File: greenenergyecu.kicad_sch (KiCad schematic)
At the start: 4 parts, among them M1 Module-vr-discrete-0.5, M2 Module-knock-0.2, M3 Module-vr-0.1, M4 Module-motor-driver-0.1

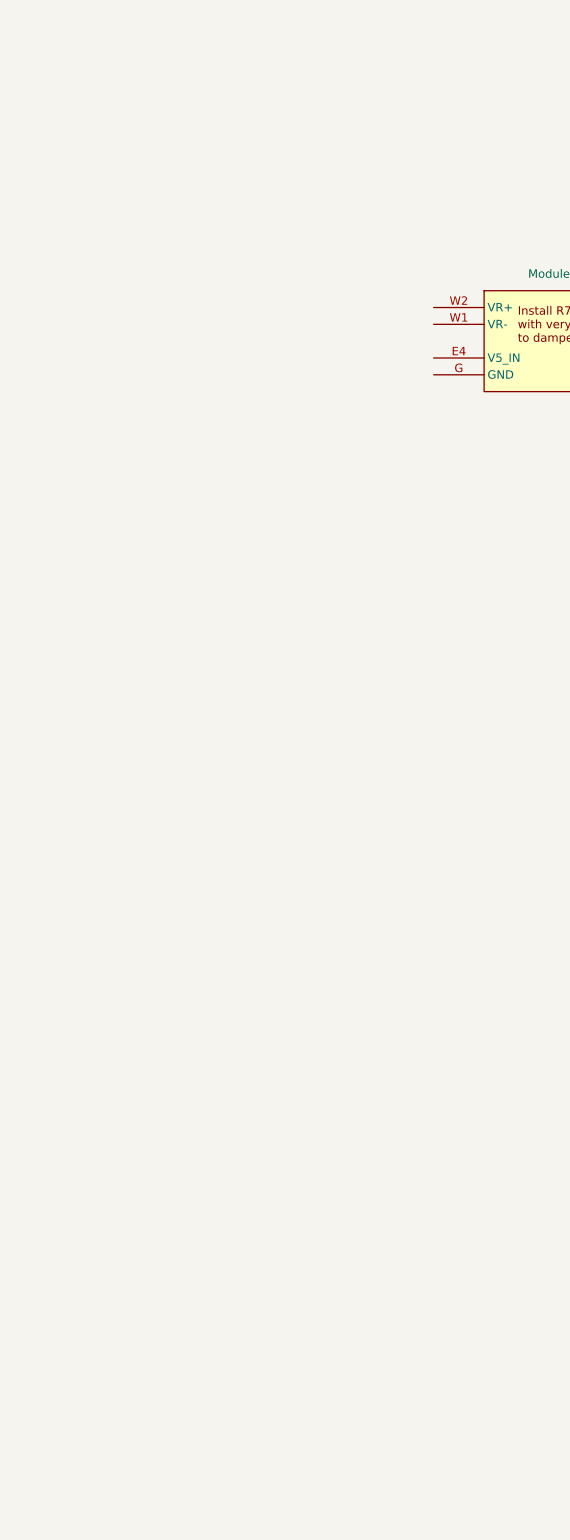
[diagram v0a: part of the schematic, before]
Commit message: ew
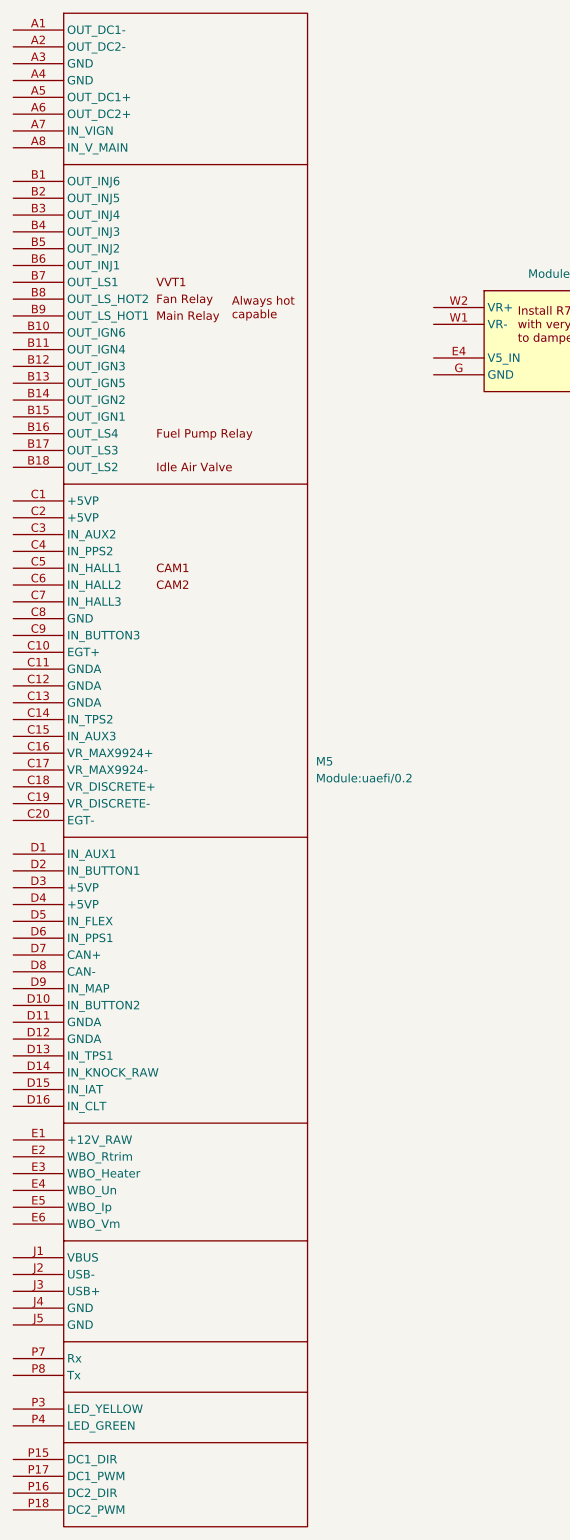
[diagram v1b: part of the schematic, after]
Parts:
- added M5: Module:uaefi/0.2, 0.2:uaefi, symbol uaefi:Module-uaefi-0.2
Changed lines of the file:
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@@
+	)
+	(symbol
+		(lib_id "uaefi:Module-uaefi-0.2")
+		(at -25.4 -3.81 0)
+		(unit 1)
+		(exclude_from_sim no)
+		(in_bom yes)
+		(on_board yes)
+		(dnp no)
+		(fields_autoplaced yes)
+		(property "Reference" "M5"
+			(at 20.32 106.6799 0)
+			(effects
+				(font
+					(size 1.27 1.27)
+				)
+				(justify left)
+			)
+		)
+		(property "Value" "Module:uaefi/0.2"
+			(at 20.32 109.2199 0)
+			(effects
+				(font
+					(size 1.27 1.27)
+				)
+				(justify left)
+			)
+		)
+		(property "Footprint" "0.2:uaefi"
+			(at -3.81 223.52 0)
+			(effects
+				(font
+					(size 1.27 1.27)
+				)
+				(hide yes)
+			)
+		)
+		(property "Datasheet" ""
+			(at -25.4 -3.81 0)
+			(effects
+				(font
+					(size 1.27 1.27)
+				)
+				(hide yes)
+			)
+		)
+		(property "Description" ""
+			(at -25.4 -3.81 0)
+			(effects
+				(font
+					(size 1.27 1.27)
+				)
+				(hide yes)
+			)
+		)
+		(pin "D12"
+		)
+		(pin "D14"
+		)
+		(pin "A1"
+		)
+		(pin "D15"
+		)
+		(pin "A6"
+		)
+		(pin "B1"
+		)
+		(pin "B11"
+		)
+		(pin "E1"
+		)
+		(pin "C17"
+		)
+		(pin "A3"
+		)
+		(pin "B16"
+		)
+		(pin "C16"
+		)
+		(pin "E2"
+		)
+		(pin "E5"
+		)
+		(pin "E6"
+		)
+		(pin "E3"
+		)
+		(pin "A7"
+		)
+		(pin "P4"
+		)
+		(pin "D3"
+		)
+		(pin "C15"
+		)
+		(pin "D4"
+		)
+		(pin "P18"
+		)
+		(pin "D8"
+		)
+		(pin "D10"
+		)
+		(pin "D16"
+		)
+		(pin "D9"
+		)
+		(pin "D6"
+		)
+		(pin "D5"
+		)
+		(pin "D7"
+		)
+		(pin "E4"
+		)
+		(pin "J1"
+		)
+		(pin "A4"
+		)
+		(pin "J3"
+		)
+		(pin "J4"
+		)
+		(pin "P16"
+		)
+		(pin "D1"
+		)
+		(pin "C19"
+		)
+		(pin "P17"
+		)
+		(pin "C20"
+		)
+		(pin "D13"
+		)
+		(pin "C18"
+		)
+		(pin "P15"
+		)
+		(pin "P3"
+		)
+		(pin "P7"
+		)
+		(pin "D11"
+		)
+		(pin "D2"
+		)
+		(pin "P8"
+		)
+		(pin "J2"
+		)
+		(pin "J5"
+		)
+		(pin "A2"
+		)
+		(pin "A5"
+		)
+		(pin "A8"
+		)
+		(pin "B10"
+		)
+		(pin "B12"
+		)
+		(pin "B13"
+		)
+		(pin "B15"
+		)
+		(pin "B14"
+		)
+		(pin "B17"
+		)
+		(pin "B18"
+		)
+		(pin "B2"
+		)
+		(pin "B3"
+		)
+		(pin "B4"
+		)
+		(pin "B5"
+		)
+		(pin "B6"
+		)
+		(pin "C11"
+		)
+		(pin "C2"
+		)
+		(pin "C5"
+		)
+		(pin "C1"
+		)
+		(pin "C8"
+		)
+		(pin "C6"
+		)
+		(pin "C12"
+		)
+		(pin "C7"
+		)
+		(pin "C9"
+		)
+		(pin "C10"
+		)
+		(pin "C4"
+		)
+		(pin "C14"
+		)
+		(pin "C13"
+		)
+		(pin "B9"
+		)
+		(pin "B7"
+		)
+		(pin "B8"
+		)
+		(pin "C3"
+		)
+		(instances
+			(project ""
+				(path "/21d7de3a-3085-4cf6-8b96-c28a6ef2f188"
+					(reference "M5")
+					(unit 1)
+				)
+			)
+		)
 	)
 	(symbol
